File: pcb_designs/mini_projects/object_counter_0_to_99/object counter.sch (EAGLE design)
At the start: 13 parts, among them IC1 4033, IC2 4033

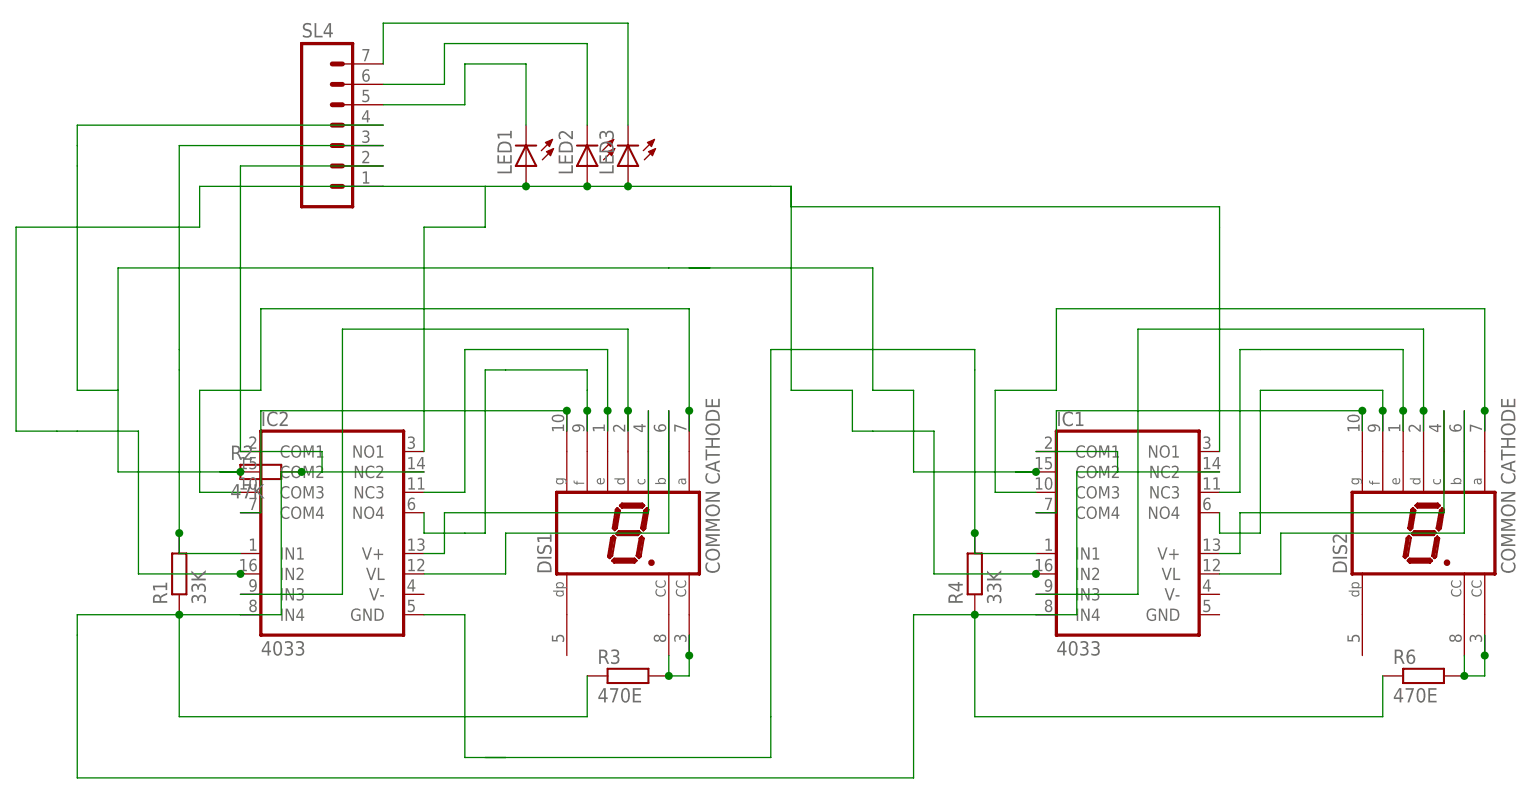
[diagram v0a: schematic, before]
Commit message: add
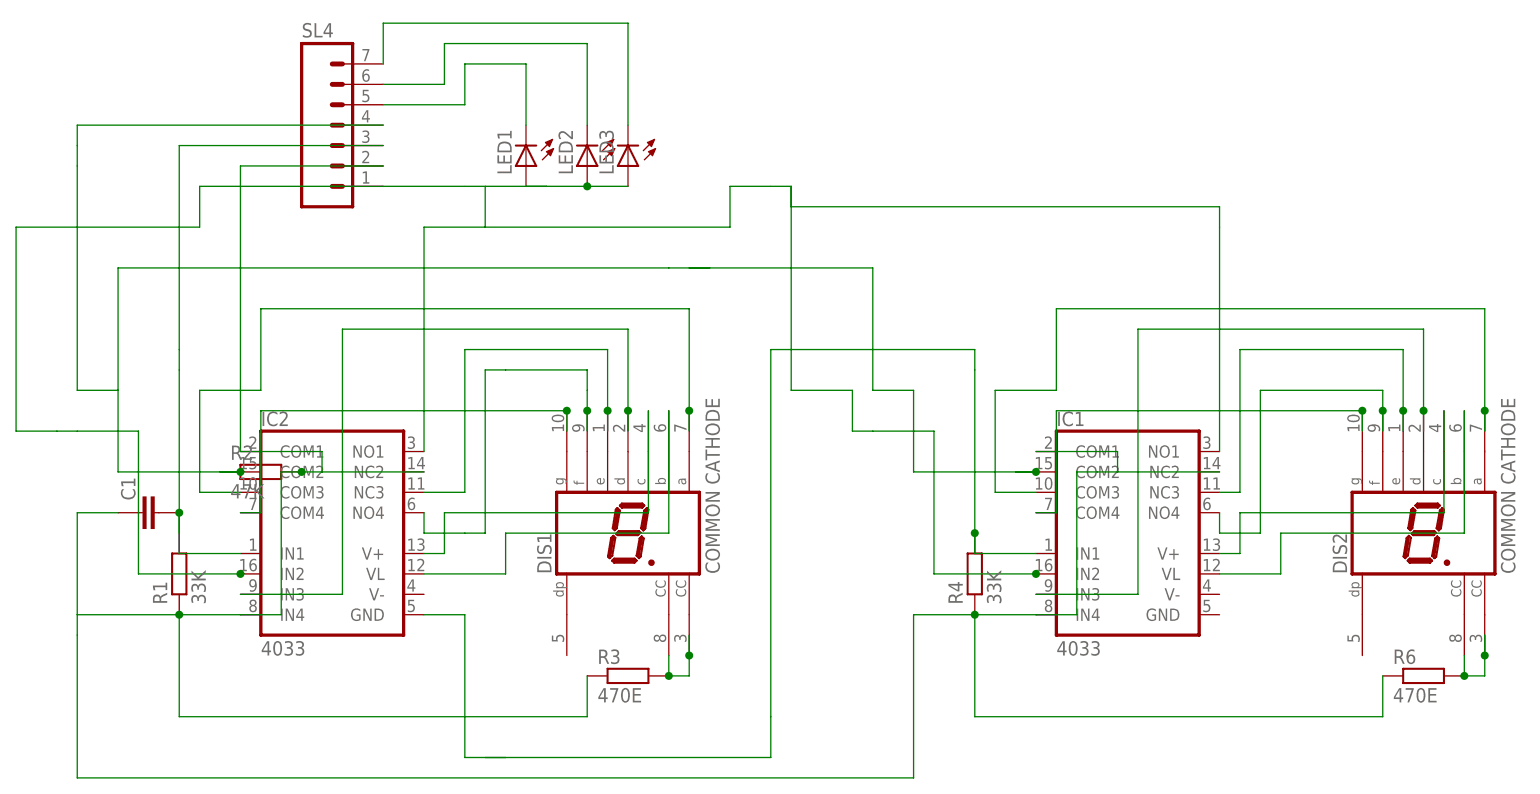
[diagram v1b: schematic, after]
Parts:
- added C1: (no value), capacitor-wima:C2,5-3
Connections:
- net N$1: now also C1.1
- net N$4: now also C1.2
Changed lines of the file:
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@@
 <?xml version="1.0" encoding="utf-8"?>
 <!DOCTYPE eagle SYSTEM "eagle.dtd">
-<eagle version="6.5.0">
+<eagle version="6.1">
 <drawing>
 <settings>
@@
 <part name="LED2" library="led" deviceset="LED" device="5MM"/>
 <part name="LED3" library="led" deviceset="LED" device="5MM"/>
+<part name="C1" library="capacitor-wima" deviceset="C" device="2,5-3"/>
 </parts>
 <sheets>
@@
 <instance part="LED2" gate="G$1" x="-40.64" y="119.38" rot="R180"/>
 <instance part="LED3" gate="G$1" x="-35.56" y="119.38" rot="R180"/>
+<instance part="C1" gate="G$1" x="-96.52" y="76.2" rot="R90"/>
 </instances>
 <busses>
@@
 <pinref part="SL4" gate="G$1" pin="2"/>
 <wire x1="-83.82" y1="119.38" x2="-66.04" y2="119.38" width="0.1524" layer="91"/>
+<pinref part="C1" gate="G$1" pin="1"/>
+<wire x1="-99.06" y1="76.2" x2="-104.14" y2="76.2" width="0.1524" layer="91"/>
+<wire x1="-104.14" y1="76.2" x2="-104.14" y2="63.5" width="0.1524" layer="91"/>
 </segment>
 </net>
@@
 <pinref part="IC2" gate="G$1" pin="IN1"/>
 <wire x1="-83.82" y1="71.12" x2="-91.44" y2="71.12" width="0.1524" layer="91"/>
-<wire x1="-91.44" y1="71.12" x2="-91.44" y2="73.66" width="0.1524" layer="91"/>
+<wire x1="-91.44" y1="71.12" x2="-91.44" y2="76.2" width="0.1524" layer="91"/>
 <pinref part="R1" gate="G$1" pin="2"/>
-<wire x1="-91.44" y1="73.66" x2="-91.44" y2="93.98" width="0.1524" layer="91"/>
-<junction x="-91.44" y="73.66"/>
+<wire x1="-91.44" y1="76.2" x2="-91.44" y2="93.98" width="0.1524" layer="91"/>
+<junction x="-91.44" y="76.2"/>
 <wire x1="-91.44" y1="93.98" x2="-91.44" y2="96.52" width="0.1524" layer="91"/>
 <wire x1="-91.44" y1="96.52" x2="-91.44" y2="121.92" width="0.1524" layer="91"/>
 <pinref part="SL4" gate="G$1" pin="3"/>
 <wire x1="-91.44" y1="121.92" x2="-66.04" y2="121.92" width="0.1524" layer="91"/>
+<pinref part="C1" gate="G$1" pin="2"/>
+<wire x1="-91.44" y1="76.2" x2="-91.44" y2="73.66" width="0.1524" layer="91"/>
 </segment>
 </net>
@@
 </segment>
 </net>
-<net name="N$2" class="0">
+<net name="N$13" class="0">
 <segment>
 <pinref part="IC2" gate="G$1" pin="NO1"/>
 <wire x1="-60.96" y1="83.82" x2="-60.96" y2="111.76" width="0.1524" layer="91"/>
 <wire x1="-60.96" y1="111.76" x2="-53.34" y2="111.76" width="0.1524" layer="91"/>
-<wire x1="-104.14" y1="86.36" x2="-96.52" y2="86.36" width="0.1524" layer="91"/>
-<wire x1="-96.52" y1="86.36" x2="-96.52" y2="68.58" width="0.1524" layer="91"/>
-<wire x1="-96.52" y1="68.58" x2="-83.82" y2="68.58" width="0.1524" layer="91"/>
-<wire x1="-104.14" y1="86.36" x2="-106.68" y2="86.36" width="0.1524" layer="91"/>
+<wire x1="-53.34" y1="111.76" x2="-53.34" y2="116.84" width="0.1524" layer="91"/>
+<pinref part="SL4" gate="G$1" pin="1"/>
+<wire x1="-66.04" y1="116.84" x2="-55.88" y2="116.84" width="0.1524" layer="91"/>
+<wire x1="-55.88" y1="116.84" x2="-53.34" y2="116.84" width="0.1524" layer="91"/>
+<wire x1="-88.9" y1="116.84" x2="-66.04" y2="116.84" width="0.1524" layer="91"/>
+<wire x1="-88.9" y1="111.76" x2="-88.9" y2="116.84" width="0.1524" layer="91"/>
 <pinref part="IC2" gate="G$1" pin="IN2"/>
 <junction x="-83.82" y="68.58"/>
+<wire x1="-96.52" y1="68.58" x2="-83.82" y2="68.58" width="0.1524" layer="91"/>
+<wire x1="-96.52" y1="86.36" x2="-96.52" y2="68.58" width="0.1524" layer="91"/>
+<wire x1="-104.14" y1="86.36" x2="-96.52" y2="86.36" width="0.1524" layer="91"/>
+<wire x1="-104.14" y1="86.36" x2="-106.68" y2="86.36" width="0.1524" layer="91"/>
 <wire x1="-106.68" y1="86.36" x2="-111.76" y2="86.36" width="0.1524" layer="91"/>
 <wire x1="-111.76" y1="86.36" x2="-111.76" y2="111.76" width="0.1524" layer="91"/>
 <wire x1="-111.76" y1="111.76" x2="-88.9" y2="111.76" width="0.1524" layer="91"/>
-<wire x1="-88.9" y1="111.76" x2="-88.9" y2="116.84" width="0.1524" layer="91"/>
-<pinref part="SL4" gate="G$1" pin="1"/>
-<wire x1="-88.9" y1="116.84" x2="-66.04" y2="116.84" width="0.1524" layer="91"/>
-<wire x1="-66.04" y1="116.84" x2="-53.34" y2="116.84" width="0.1524" layer="91"/>
-<wire x1="-53.34" y1="116.84" x2="-48.26" y2="116.84" width="0.1524" layer="91"/>
-<wire x1="-48.26" y1="116.84" x2="-40.64" y2="116.84" width="0.1524" layer="91"/>
-<wire x1="-40.64" y1="116.84" x2="-35.56" y2="116.84" width="0.1524" layer="91"/>
-<wire x1="-53.34" y1="111.76" x2="-53.34" y2="116.84" width="0.1524" layer="91"/>
-<wire x1="-35.56" y1="116.84" x2="-17.78" y2="116.84" width="0.1524" layer="91"/>
+<wire x1="-53.34" y1="111.76" x2="-22.86" y2="111.76" width="0.1524" layer="91"/>
+<wire x1="-22.86" y1="111.76" x2="-22.86" y2="116.84" width="0.1524" layer="91"/>
 <pinref part="IC1" gate="G$1" pin="IN2"/>
 <junction x="15.24" y="68.58"/>
@@
 <wire x1="-17.78" y1="116.84" x2="-15.24" y2="116.84" width="0.1524" layer="91"/>
 <wire x1="-15.24" y1="116.84" x2="-15.24" y2="114.3" width="0.1524" layer="91"/>
-<pinref part="LED1" gate="G$1" pin="A"/>
-<junction x="-48.26" y="116.84"/>
+<wire x1="-22.86" y1="116.84" x2="-17.78" y2="116.84" width="0.1524" layer="91"/>
+<pinref part="LED3" gate="G$1" pin="A"/>
+<wire x1="-40.64" y1="116.84" x2="-35.56" y2="116.84" width="0.1524" layer="91"/>
 <pinref part="LED2" gate="G$1" pin="A"/>
 <junction x="-40.64" y="116.84"/>
-<pinref part="LED3" gate="G$1" pin="A"/>
-<junction x="-35.56" y="116.84"/>
-</segment>
-</net>
+<wire x1="-48.26" y1="116.84" x2="-45.72" y2="116.84" width="0.1524" layer="91"/>
+<pinref part="LED1" gate="G$1" pin="A"/>
+<wire x1="-45.72" y1="116.84" x2="-40.64" y2="116.84" width="0.1524" layer="91"/>
+<wire x1="-53.34" y1="116.84" x2="-45.72" y2="116.84" width="0.1524" layer="91"/>
+</segment>
+</net>
